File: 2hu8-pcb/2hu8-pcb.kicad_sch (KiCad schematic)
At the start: 1 part, among them U1 ProMicro

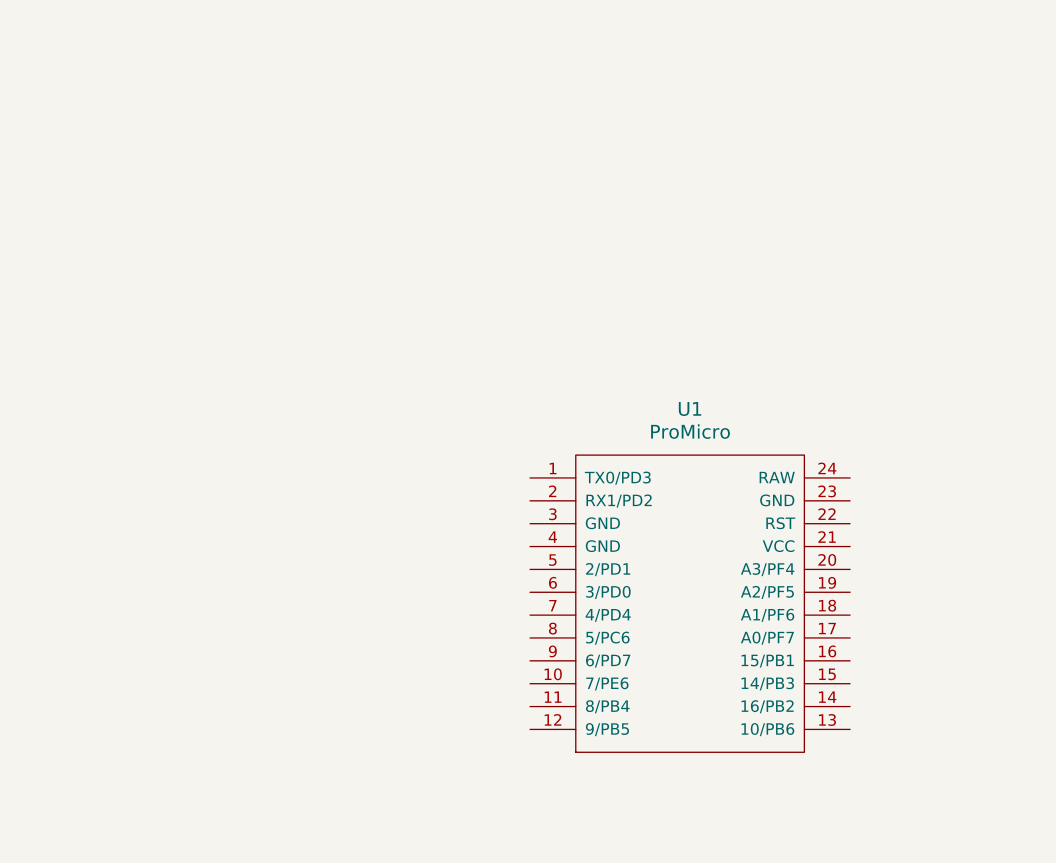
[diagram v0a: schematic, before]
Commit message: start schematic
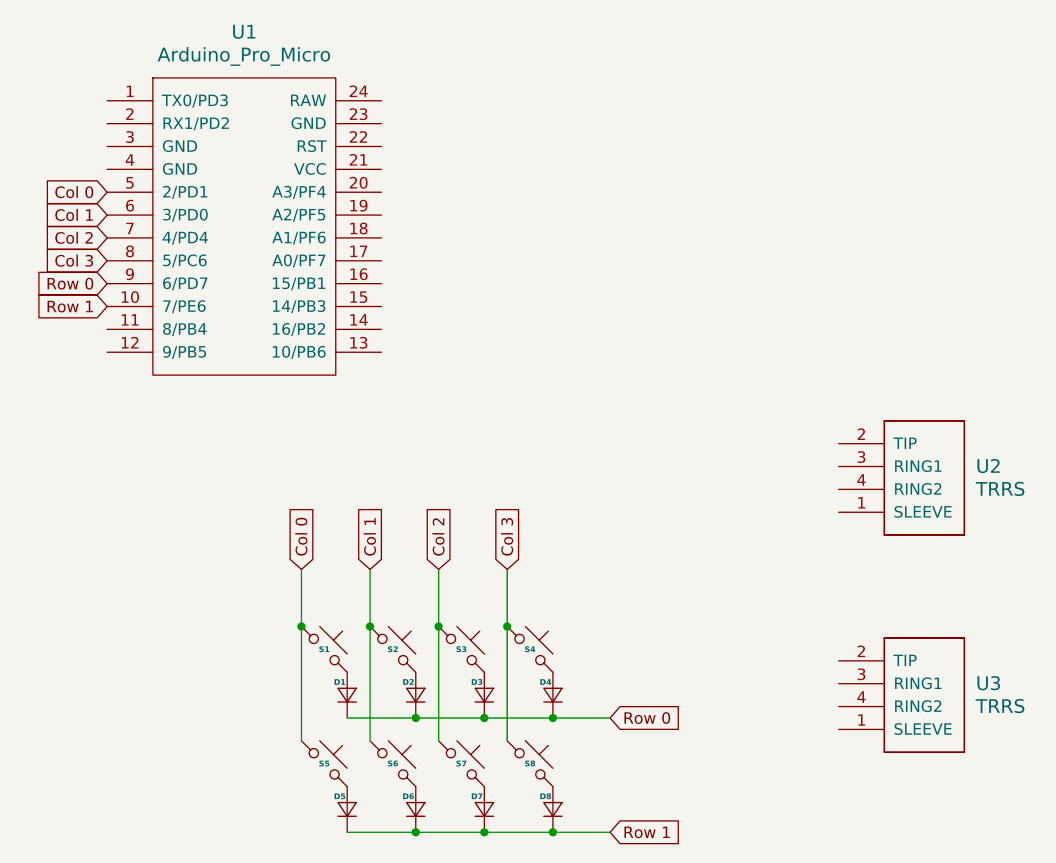
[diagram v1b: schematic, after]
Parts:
- removed U1: ProMicro, symbol keebio:ProMicro
- added D1, D2, D3, D4, D5, D6, D7, D8: (no value), ScottoKeebs_Components:Diode_DO-35, symbol ScottoKeebs:Placeholder_Diode
- added S1, S2, S3, S4, S5, S6, S7, S8: (no value), Button_Switch_Keyboard:SW_Cherry_MX_1.00u_PCB, symbol ScottoKeebs:Placeholder_Keyswitch
- added U1: Arduino_Pro_Micro, ScottoKeebs_MCU:Arduino_Pro_Micro, symbol ScottoKeebs:MCU_Arduino_Pro_Micro
- added U2, U3: TRRS, ScottoKeebs_Components:TRRS_PJ-320A, symbol ScottoKeebs:Placeholder_TRRS
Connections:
- new net: D5.2 (A), S5.2
- new net: D2.2 (A), S2.2
- new net: D1.2 (A), S1.2
- new net: D3.2 (A), S3.2
- new net: D6.2 (A), S6.2
- new net: D8.2 (A), S8.2
- new net: D7.2 (A), S7.2
- new net: D4.2 (A), S4.2
- new net Col 0: S1.1, S5.1, U1.5 (2/PD1)
- new net Col 1: S2.1, S6.1, U1.6 (3/PD0)
- new net Col 2: S3.1, S7.1, U1.7 (4/PD4)
- new net Col 3: S4.1, S8.1, U1.8 (5/PC6)
- new net Row 0: D1.1 (K), D2.1 (K), D3.1 (K), D4.1 (K), U1.9 (6/PD7)
- new net Row 1: D5.1 (K), D6.1 (K), D7.1 (K), D8.1 (K), U1.10 (7/PE6)
